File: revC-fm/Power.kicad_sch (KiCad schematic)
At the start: 65 parts, among them P2 TSM-102-01-L-SV-P-TR, Q1 MMDT5551-7-F, Q2 MMDT5551-7-F, SW3 SW_SPST, SW4 SW_SPST, SW5 SW_SPST, SW6 SW_SPST, U10 INA226A, U12 TPS54226PWPR, U13 BQ25883RGER, U14 INA226A, U15 INA226A, U43 INA226A, U45 INA226A, U9 ADM1176-1ARMZ-R7

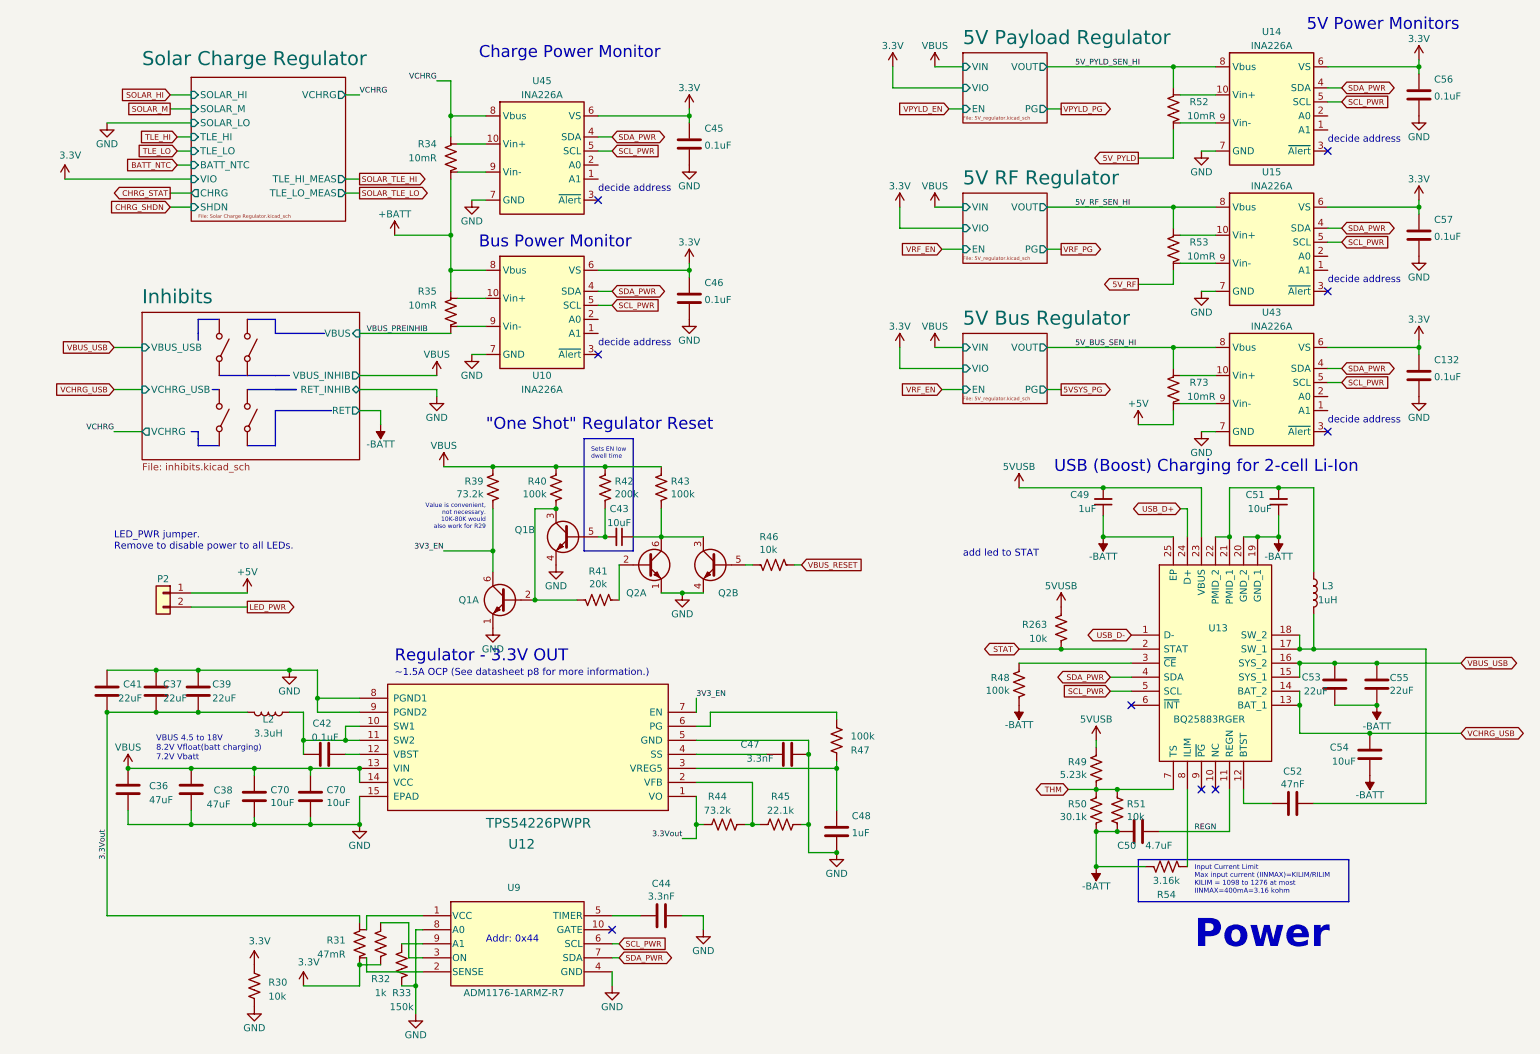
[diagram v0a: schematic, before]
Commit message: routing
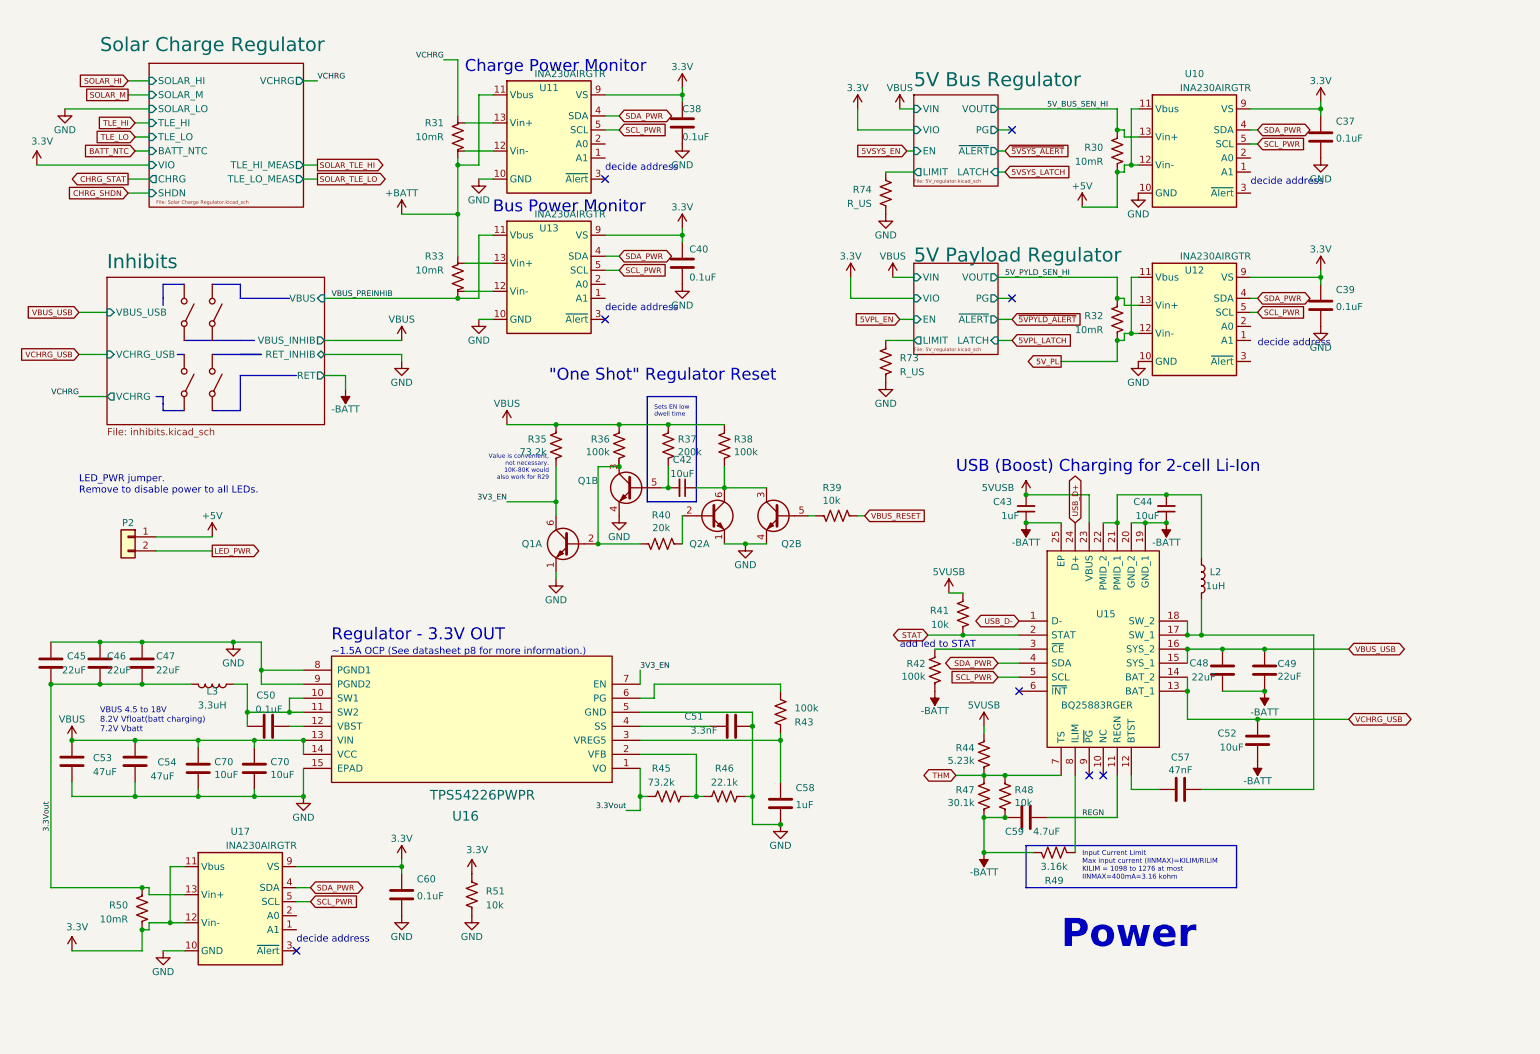
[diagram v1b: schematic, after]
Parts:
- removed C44: 3.3nF, Capacitor_SMD:C_0402_1005Metric, symbol Device:C
- removed C57: 0.1uF, Capacitor_SMD:C_0402_1005Metric, symbol Device:C
- removed R32: 1k, Resistor_SMD:R_0603_1608Metric, symbol Device:R_US
- removed R33: 150k, Resistor_SMD:R_0603_1608Metric, symbol Device:R_US
- removed R53: 10mR, SierraLobo:KRL3216, symbol SierraLobo:R_US_SENSE
- removed U15: INA226A, Package_SO:VSSOP-10_3x3mm_P0.5mm, symbol SierraLobo:INA226A
- removed U9: ADM1176-1ARMZ-R7, SierraLobo:ADM1176-1ARMZ-R7, symbol SierraLobo:ADM1176-1ARMZ-R7
- added C60: 0.1uF, Capacitor_SMD:C_0603_1608Metric, symbol Device:C
- added R73, R74: R_US, Resistor_SMD:R_0603_1608Metric, symbol Device:R_US
- added U17: INA230AIRGTR, Package_DFN_QFN:VQFN-16-1EP_3x3mm_P0.5mm_EP1.68x1.68mm, symbol SierraLobo:INA230AxRGT
- C37: renamed from C132; footprint Capacitor_SMD:C_0402_1005Metric -> Capacitor_SMD:C_0603_1608Metric
- C38: renamed from C45; footprint Capacitor_SMD:C_0402_1005Metric -> Capacitor_SMD:C_0603_1608Metric
- C39: renamed from C56; footprint Capacitor_SMD:C_0402_1005Metric -> Capacitor_SMD:C_0603_1608Metric
- C40: renamed from C46; footprint Capacitor_SMD:C_0402_1005Metric -> Capacitor_SMD:C_0603_1608Metric
- C50: renamed from C42; footprint Capacitor_SMD:C_0402_1005Metric -> Capacitor_SMD:C_0603_1608Metric
- C51: renamed from C47; footprint Capacitor_SMD:C_0402_1005Metric -> Capacitor_SMD:C_0603_1608Metric
- C57: renamed from C52; footprint Capacitor_SMD:C_0402_1005Metric -> Capacitor_SMD:C_0603_1608Metric
- R30: renamed from R73; footprint SierraLobo:KRL3216 -> Resistor_SMD:R_1210_3225Metric; symbol SierraLobo:R_US_SENSE -> Device:R_US
- R32: renamed from R52; footprint SierraLobo:KRL3216 -> Resistor_SMD:R_1210_3225Metric; symbol SierraLobo:R_US_SENSE -> Device:R_US
- R50: renamed from R31; value 47mR -> 10mR; footprint SierraLobo:KRL3216 -> Resistor_SMD:R_1210_3225Metric; symbol SierraLobo:R_US_SENSE -> Device:R_US
- U10: renamed from U43; value INA226A -> INA230AIRGTR; footprint Package_SO:VSSOP-10_3x3mm_P0.5mm -> Package_DFN_QFN:VQFN-16-1EP_3x3mm_P0.5mm_EP1.68x1.68mm; symbol SierraLobo:INA226A -> SierraLobo:INA230AxRGT
- U11: renamed from U45; value INA226A -> INA230AIRGTR; footprint Package_SO:VSSOP-10_3x3mm_P0.5mm -> Package_DFN_QFN:VQFN-16-1EP_3x3mm_P0.5mm_EP1.68x1.68mm; symbol SierraLobo:INA226A -> SierraLobo:INA230AxRGT
- U12: renamed from U14; value INA226A -> INA230AIRGTR; footprint Package_SO:VSSOP-10_3x3mm_P0.5mm -> Package_DFN_QFN:VQFN-16-1EP_3x3mm_P0.5mm_EP1.68x1.68mm; symbol SierraLobo:INA226A -> SierraLobo:INA230AxRGT
- U13: renamed from U10; value INA226A -> INA230AIRGTR; footprint Package_SO:VSSOP-10_3x3mm_P0.5mm -> Package_DFN_QFN:VQFN-16-1EP_3x3mm_P0.5mm_EP1.68x1.68mm; symbol SierraLobo:INA226A -> SierraLobo:INA230AxRGT
- renumbered C43 to C42, C49 to C43, C51 to C44, C41 to C45, C37 to C46, C39 to C47, C53 to C48, C55 to C49, C54 to C52, C36 to C53, C38 to C54, C48 to C58, C50 to C59, L3 to L2, L2 to L3, R34 to R31, R35 to R33, R39 to R35, R40 to R36, R42 to R37, R43 to R38, R46 to R39, R41 to R40, R263 to R41, R48 to R42, R47 to R43, R49 to R44, R44 to R45, R45 to R46, R50 to R47, R51 to R48, R54 to R49, R30 to R51, SW5 to SW4, SW4 to SW5, U13 to U15, U12 to U16
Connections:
- net +5V: now also U10.11 (Vbus), U10.12 (Vin-); no longer C43.2, R41.2, R44.1, U15.23 (VBUS)
- net +BATT: now also U11.11 (Vbus); no longer U13.8 (Vbus)
- net 3.3V: now also U10.9 (VS), U11.9 (VS), U12.9 (VS), U13.9 (VS), C60.1, U17.11 (Vbus), U17.12 (Vin-), U17.9 (VS); no longer U10.6 (VS), U11.6 (VS), U12.6 (VS), U13.6 (VS)
- net 3.3Vout: now also U17.13 (Vin+)
- net 5V_BUS_SEN_HI: now also U10.13 (Vin+); no longer U10.8 (Vbus)
- net 5V_PYLD_SEN_HI: now also U12.13 (Vin+); no longer U12.8 (Vbus)
- net SCL_PWR: now also U17.5 (SCL)
- net SDA_PWR: now also U17.4 (SDA)
- net VBUS_PREINHIB: now also U13.11 (Vbus)
- net VCHRG: no longer U11.8 (Vbus)
- net at R33.3: now also U13.12 (Vin-); no longer U13.9 (Vin-)
- net at R33.4: now also U13.13 (Vin+); no longer U13.10 (Vin+)
- net at R31.3: now also U11.12 (Vin-); no longer U11.9 (Vin-)
- net at R31.4: now also U11.13 (Vin+); no longer U11.10 (Vin+)
- net EP: now reaches U12.10 (GND)
- net EP: now also C37.2, C38.2, C39.2, C40.2, C45.1, C46.1, C47.1, C51.2, C53.2, C54.2, C58.2, C70.2, C70.2, Q1.1 (E1), Q1.4 (E2), Q2.1 (E1), Q2.4 (E2), R46.1, R51.2, U10.10 (GND), U10.17 (EP), U11.10 (GND), U11.17 (EP), U12.17 (EP), U13.10 (GND), U13.17 (EP), U16.15 (EPAD), U16.5 (GND), U16.8 (PGND1), U16.9 (PGND2), C60.2, R73.2, R74.2, U17.10 (GND), U17.17 (EP); no longer R32.4
- net 5V_PYLD renamed 5V_PL
- net 5V_PL: now also U12.11 (Vbus), U12.12 (Vin-)
- removed net GND: C37.2, C38.2, C39.2, C40.2, C45.1, C46.1, C47.1, C51.2, C53.2, C54.2, C58.2, C70.2, C70.2, Q1.1 (E1), Q1.4 (E2), Q2.1 (E1), Q2.4 (E2), R46.1, R51.2, U10.7 (GND), U11.7 (GND), U12.7 (GND), U13.7 (GND), U16.15 (EPAD), U16.5 (GND), U16.8 (PGND1), U16.9 (PGND2)
- new net 5V Bus Regulator/LIMIT: R74.1
- new net 5V Payload Regulator/LIMIT: R73.1
- new net 5VUSB: C43.2, R41.2, R44.1, U15.23 (VBUS)
- no-connect marks 9 -> 8
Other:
- removed sheet 5V RF Regulator
- sheet 5V Bus Regulator ports: added LATCH, LIMIT, ~{ALERT}; removed none
- sheet 5V Payload Regulator ports: added LATCH, LIMIT, ~{ALERT}; removed none
- note removed: "5V Power Monitors"
- note removed: "Addr: 0x44"
- moved on the sheet: C37, C38, C39, C40, C42, C43, C44, C45, C46, C47, C48, C49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
